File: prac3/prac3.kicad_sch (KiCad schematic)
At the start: 5 parts, among them J1 Screw_Terminal_01x07, SW1 SW_Push

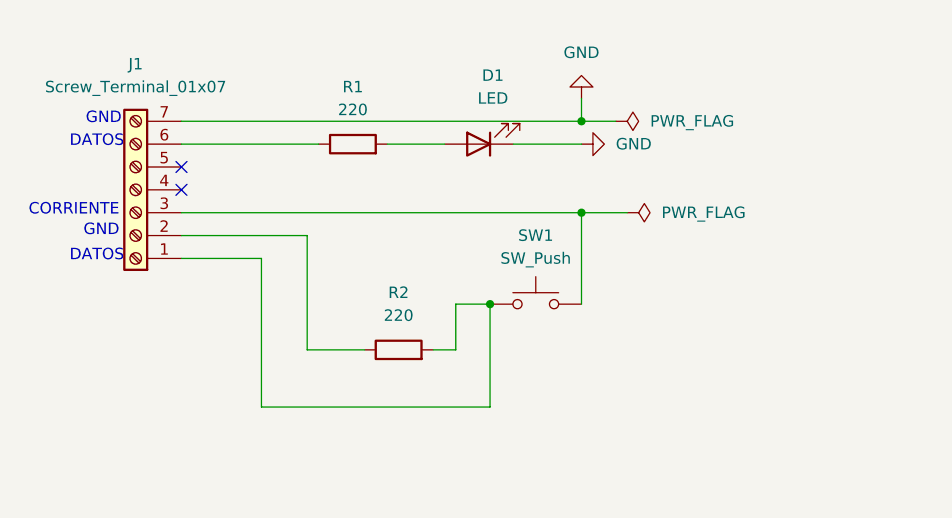
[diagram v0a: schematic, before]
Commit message: prac3 2do parcial
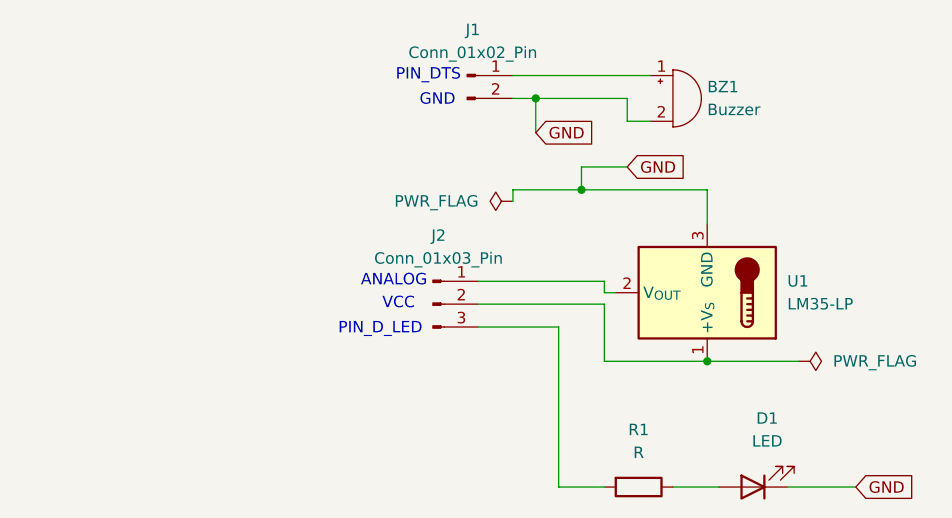
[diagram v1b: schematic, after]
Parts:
- removed J1: Screw_Terminal_01x07, TerminalBlock_Phoenix:TerminalBlock_Phoenix_MKDS-1,5-7_1x07_P5.00mm_Horizontal, symbol Connector:Screw_Terminal_01x07
- removed R2: 220, Resistor_SMD:R_0805_2012Metric, symbol Device:R
- removed SW1: SW_Push, Button_Switch_SMD:SW_Push_1P1T_NO_CK_KMR2, symbol Switch:SW_Push
- added BZ1: Buzzer, Buzzer_Beeper:Buzzer_15x7.5RM7.6, symbol Device:Buzzer
- added J1: Conn_01x02_Pin, Connector_PinHeader_2.54mm:PinHeader_1x02_P2.54mm_Vertical, symbol Connector:Conn_01x02_Pin
- added J2: Conn_01x03_Pin, Connector_PinHeader_2.54mm:PinHeader_1x03_P2.54mm_Vertical, symbol Connector:Conn_01x03_Pin
- added U1: LM35-LP, Package_TO_SOT_THT:TO-92_Inline, symbol Sensor_Temperature:LM35-LP
- R1: value 220 -> R
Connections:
- net GND: now also BZ1.2 (-), J1.2 (Pin_2), U1.3 (GND)
- net at D1.2 (A): now also R1.1; no longer R1.2
- new net: J2.3 (Pin_3), R1.2
- new net: J2.2 (Pin_2), U1.1 (+V_{S})
- new net: J2.1 (Pin_1), U1.2 (V_{OUT})
- new net: BZ1.1 (+), J1.1 (Pin_1)
- no-connect marks 2 -> 0
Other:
- note added: "ANALOG"
- note added: "PIN_DTS"
- note added: "PIN_D_LED"
- note added: "VCC"
- note removed: "CORRIENTE"
- note removed: "DATOS"
